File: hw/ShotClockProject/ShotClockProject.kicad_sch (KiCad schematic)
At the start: 5 parts, among them SW5 SW_SPDT

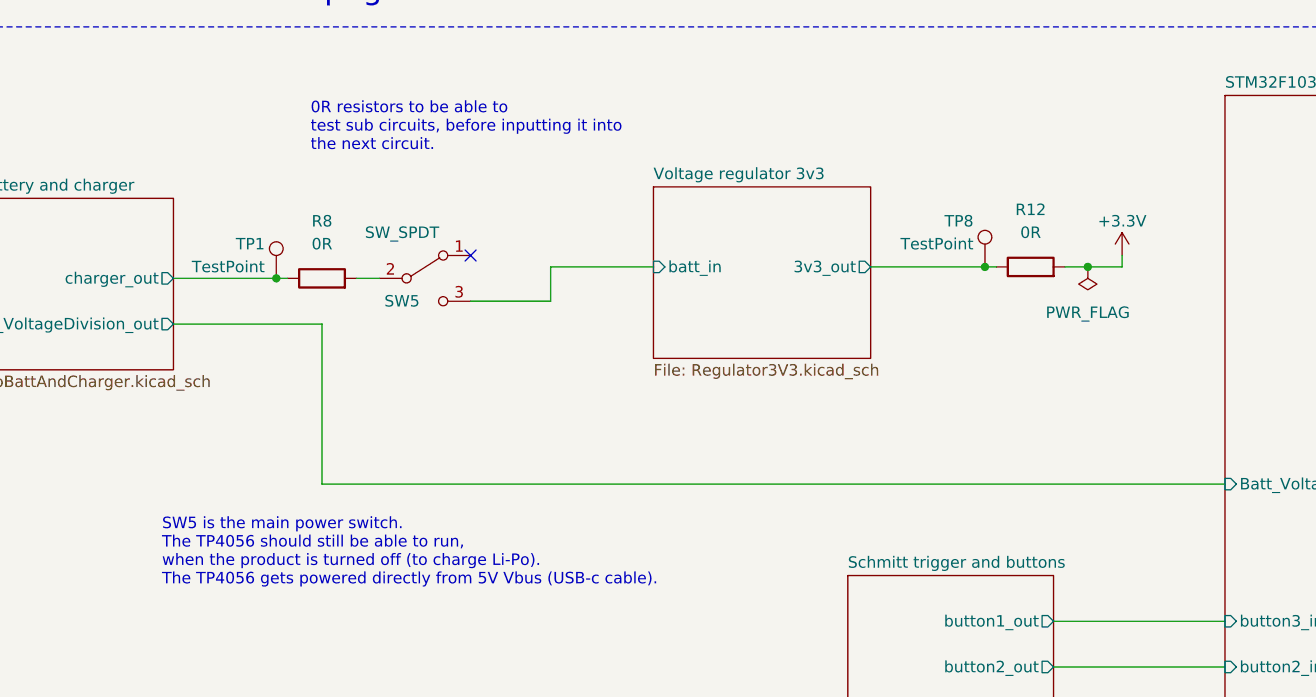
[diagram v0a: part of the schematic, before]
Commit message: Renamed references
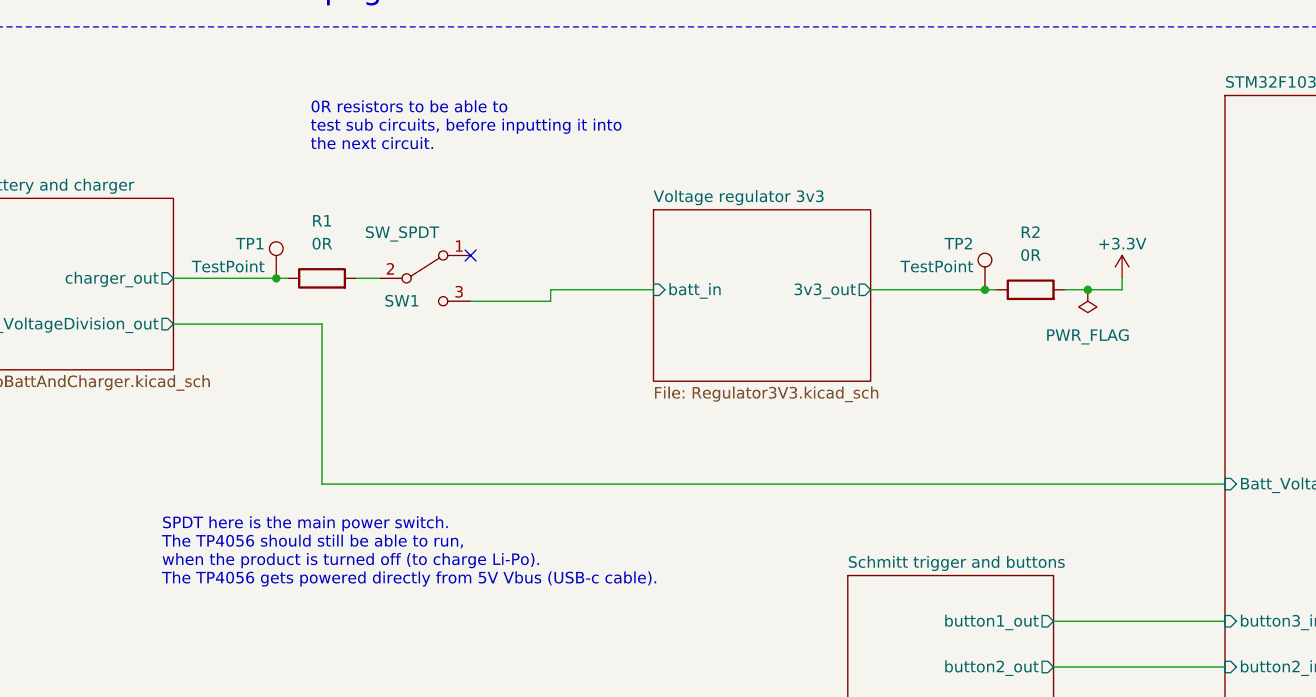
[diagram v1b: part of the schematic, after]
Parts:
- renumbered R8 to R1, R12 to R2, SW5 to SW1, TP8 to TP2
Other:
- note added: "SPDT here is the main power switch. The TP4056 should still be able to run, when the product is turned off (to charge Li-Po). The TP4056 gets powered directly from 5V Vbus (USB-c cable)."
- note removed: "SW5 is the main power switch. The TP4056 should still be able to run, when the product is turned off (to charge Li-Po). The TP4056 gets powered directly from 5V Vbus (USB-c cable)."
- moved on the sheet: R2, TP2
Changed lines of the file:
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@@
   (junction (at 59.69 49.53) (diameter 0) (color 0 0 0 0)
   )
-  (junction (at 149.86 48.26) (diameter 0) (color 0 0 0 0)
-  )
-  (junction (at 138.43 48.26) (diameter 0) (color 0 0 0 0)
+  (junction (at 149.86 50.8) (diameter 0) (color 0 0 0 0)
+  )
+  (junction (at 138.43 50.8) (diameter 0) (color 0 0 0 0)
   )
   (no_connect (at 81.28 46.99))
@@
     (stroke (width 0) (type default))
   )
-  (wire (pts (xy 138.43 48.26) (xy 139.7 48.26))
+  (wire (pts (xy 138.43 50.8) (xy 139.7 50.8))
     (stroke (width 0) (type default))
   )
@@
     (stroke (width 0) (type default))
   )
-  (wire (pts (xy 90.17 48.26) (xy 101.6 48.26))
+  (wire (pts (xy 90.17 50.8) (xy 90.17 52.07))
     (stroke (width 0) (type default))
   )
@@
     (stroke (width 0) (type default))
   )
-  (wire (pts (xy 125.73 48.26) (xy 138.43 48.26))
+  (wire (pts (xy 125.73 50.8) (xy 138.43 50.8))
     (stroke (width 0) (type default))
   )
@@
     (stroke (width 0) (type default))
   )
-  (wire (pts (xy 153.67 48.26) (xy 153.67 46.99))
+  (wire (pts (xy 153.67 50.8) (xy 153.67 49.53))
     (stroke (width 0) (type default))
   )
@@
     (stroke (width 0) (type default))
   )
-  (wire (pts (xy 147.32 48.26) (xy 149.86 48.26))
+  (wire (pts (xy 147.32 50.8) (xy 149.86 50.8))
     (stroke (width 0) (type default))
   )
@@
     (stroke (width 0) (type default))
   )
-  (wire (pts (xy 90.17 52.07) (xy 90.17 48.26))
-    (stroke (width 0) (type default))
-  )
   (wire (pts (xy 203.2 78.74) (xy 231.14 78.74))
     (stroke (width 0) (type default))
   )
-  (wire (pts (xy 149.86 48.26) (xy 153.67 48.26))
+  (wire (pts (xy 149.86 50.8) (xy 153.67 50.8))
+    (stroke (width 0) (type default))
+  )
+  (wire (pts (xy 101.6 50.8) (xy 90.17 50.8))
     (stroke (width 0) (type default))
   )
@@
     (effects (font (size 2.5 2.5) (color 255 0 0 1)) (justify left bottom))
   )
-  (text "SW5 is the main power switch.\nThe TP4056 should still be able to run, \nwhen the product is turned off (to charge Li-Po).\nThe TP4056 gets powered directly from 5V Vbus (USB-c cable)."
+  (text "SPDT here is the main power switch.\nThe TP4056 should still be able to run, \nwhen the product is turned off (to charge Li-Po).\nThe TP4056 gets powered directly from 5V Vbus (USB-c cable)."
     (at 46.99 83.82 0)
     (effects (font (size 1.27 1.27)) (justify left bottom))
@@
   (symbol (lib_id "Switch:SW_SPDT") (at 76.2 49.53 0) (unit 1)
     (in_bom yes) (on_board yes) (dnp no)
-    (property "Reference" "SW5" (at 73.66 52.07 0)
+    (property "Reference" "SW1" (at 73.66 52.07 0)
       (effects (font (size 1.27 1.27)))
     )
@@
       (project "ShotClockProject"
         (path "/5fd859aa-754d-49c2-9762-3f7ebe3bb64c"
-          (reference "SW5") (unit 1)
+          (reference "SW1") (unit 1)
         )
         (path "/5fd859aa-754d-49c2-9762-3f7ebe3bb64c/d53b1cd8-24cb-4dc0-9a02-0cd96c1f4291"
@@
   (symbol (lib_id "Device:R") (at 64.77 49.53 90) (unit 1)
     (in_bom yes) (on_board yes) (dnp no) (fields_autoplaced)
-    (property "Reference" "R8" (at 64.77 43.18 90)
+    (property "Reference" "R1" (at 64.77 43.18 90)
       (effects (font (size 1.27 1.27)))
     )
@@
       (project "ShotClockProject"
         (path "/5fd859aa-754d-49c2-9762-3f7ebe3bb64c"
-          (reference "R8") (unit 1)
-        )
-      )
-    )
-  )
-  (symbol (lib_id "Connector:TestPoint") (at 138.43 48.26 0) (mirror y) (unit 1)
+          (reference "R1") (unit 1)
+        )
+      )
+    )
+  )
+  (symbol (lib_id "Connector:TestPoint") (at 138.43 50.8 0) (mirror y) (unit 1)
     (in_bom yes) (on_board yes) (dnp no)
-    (property "Reference" "TP8" (at 137.16 43.18 0)
-      (effects (font (size 1.27 1.27)) (justify left))
-    )
-    (property "Value" "TestPoint" (at 137.16 45.72 0)
-      (effects (font (size 1.27 1.27)) (justify left))
-    )
-    (property "Footprint" "TestPoint:TestPoint_Pad_D2.5mm" (at 133.35 48.26 0)
-      (effects (font (size 1.27 1.27)) hide)
-    )
-    (property "Datasheet" "~" (at 133.35 48.26 0)
-      (effects (font (size 1.27 1.27)) hide)
-    )
-    (pin "1")
-    (instances
-      (project "ShotClockProject"
-        (path "/5fd859aa-754d-49c2-9762-3f7ebe3bb64c"
-          (reference "TP8") (unit 1)
+    (property "Reference" "TP2" (at 137.16 45.72 0)
+      (effects (font (size 1.27 1.27)) (justify left))
+    )
+    (property "Value" "TestPoint" (at 137.16 48.26 0)
+      (effects (font (size 1.27 1.27)) (justify left))
+    )
+    (property "Footprint" "TestPoint:TestPoint_Pad_D2.5mm" (at 133.35 50.8 0)
+      (effects (font (size 1.27 1.27)) hide)
+    )
+    (property "Datasheet" "~" (at 133.35 50.8 0)
+      (effects (font (size 1.27 1.27)) hide)
+    )
+    (pin "1")
+    (instances
+      (project "ShotClockProject"
+        (path "/5fd859aa-754d-49c2-9762-3f7ebe3bb64c"
+          (reference "TP2") (unit 1)
         )
         (path "/5fd859aa-754d-49c2-9762-3f7ebe3bb64c/17367eb9-0f4d-4017-b1ca-d50430410a5d"
@@
     )
   )
-  (symbol (lib_id "Device:R") (at 143.51 48.26 90) (unit 1)
+  (symbol (lib_id "Device:R") (at 143.51 50.8 90) (unit 1)
     (in_bom yes) (on_board yes) (dnp no) (fields_autoplaced)
-    (property "Reference" "R12" (at 143.51 41.91 90)
-      (effects (font (size 1.27 1.27)))
-    )
-    (property "Value" "0R" (at 143.51 44.45 90)
-      (effects (font (size 1.27 1.27)))
-    )
-    (property "Footprint" "Resistor_SMD:R_0603_1608Metric" (at 143.51 50.038 90)
-      (effects (font (size 1.27 1.27)) hide)
-    )
-    (property "Datasheet" "~" (at 143.51 48.26 0)
+    (property "Reference" "R2" (at 143.51 44.45 90)
+      (effects (font (size 1.27 1.27)))
+    )
+    (property "Value" "0R" (at 143.51 46.99 90)
+      (effects (font (size 1.27 1.27)))
+    )
+    (property "Footprint" "Resistor_SMD:R_0603_1608Metric" (at 143.51 52.578 90)
+      (effects (font (size 1.27 1.27)) hide)
+    )
+    (property "Datasheet" "~" (at 143.51 50.8 0)
       (effects (font (size 1.27 1.27)) hide)
     )
@@
       (project "ShotClockProject"
         (path "/5fd859aa-754d-49c2-9762-3f7ebe3bb64c"
-          (reference "R12") (unit 1)
-        )
-      )
-    )
-  )
-  (symbol (lib_id "power:PWR_FLAG") (at 149.86 48.26 180) (unit 1)
+          (reference "R2") (unit 1)
+        )
+      )
+    )
+  )
+  (symbol (lib_id "power:PWR_FLAG") (at 149.86 50.8 180) (unit 1)
     (in_bom yes) (on_board yes) (dnp no) (fields_autoplaced)
-    (property "Reference" "#FLG02" (at 149.86 50.165 0)
-      (effects (font (size 1.27 1.27)) hide)
-    )
-    (property "Value" "PWR_FLAG" (at 149.86 53.34 0)
-      (effects (font (size 1.27 1.27)))
-    )
-    (property "Footprint" "" (at 149.86 48.26 0)
-      (effects (font (size 1.27 1.27)) hide)
-    )
-    (property "Datasheet" "~" (at 149.86 48.26 0)
+    (property "Reference" "#FLG02" (at 149.86 52.705 0)
+      (effects (font (size 1.27 1.27)) hide)
+    )
+    (property "Value" "PWR_FLAG" (at 149.86 55.88 0)
+      (effects (font (size 1.27 1.27)))
+    )
+    (property "Footprint" "" (at 149.86 50.8 0)
+      (effects (font (size 1.27 1.27)) hide)
+    )
+    (property "Datasheet" "~" (at 149.86 50.8 0)
       (effects (font (size 1.27 1.27)) hide)
     )
@@
         )
         (path "/5fd859aa-754d-49c2-9762-3f7ebe3bb64c"
-          (reference "#FLG03") (unit 1)
-        )
-      )
-    )
-  )
-  (symbol (lib_id "power:+3.3V") (at 153.67 46.99 0) (unit 1)
+          (reference "#FLG01") (unit 1)
+        )
+      )
+    )
+  )
+  (symbol (lib_id "power:+3.3V") (at 153.67 49.53 0) (unit 1)
     (in_bom yes) (on_board yes) (dnp no)
-    (property "Reference" "#PWR033" (at 153.67 50.8 0)
-      (effects (font (size 1.27 1.27)) hide)
-    )
-    (property "Value" "+3.3V" (at 153.67 43.18 0)
-      (effects (font (size 1.27 1.27)))
-    )
-    (property "Footprint" "" (at 153.67 46.99 0)
-      (effects (font (size 1.27 1.27)) hide)
-    )
-    (property "Datasheet" "" (at 153.67 46.99 0)
-      (effects (font (size 1.27 1.27)) hide)
-    )
-    (pin "1")
-    (instances
-      (project "ShotClockProject"
-        (path "/5fd859aa-754d-49c2-9762-3f7ebe3bb64c"
-          (reference "#PWR033") (unit 1)
+    (property "Reference" "#PWR01" (at 153.67 53.34 0)
+      (effects (font (size 1.27 1.27)) hide)
+    )
+    (property "Value" "+3.3V" (at 153.67 45.72 0)
+      (effects (font (size 1.27 1.27)))
+    )
+    (property "Footprint" "" (at 153.67 49.53 0)
+      (effects (font (size 1.27 1.27)) hide)
+    )
+    (property "Datasheet" "" (at 153.67 49.53 0)
+      (effects (font (size 1.27 1.27)) hide)
+    )
+    (pin "1")
+    (instances
+      (project "ShotClockProject"
+        (path "/5fd859aa-754d-49c2-9762-3f7ebe3bb64c"
+          (reference "#PWR01") (unit 1)
         )
         (path "/5fd859aa-754d-49c2-9762-3f7ebe3bb64c/d53b1cd8-24cb-4dc0-9a02-0cd96c1f4291"
@@
     )
   )
-  (sheet (at 101.6 39.37) (size 24.13 19.05) (fields_autoplaced)
+  (sheet (at 101.6 41.91) (size 24.13 19.05) (fields_autoplaced)
     (stroke (width 0.1524) (type solid))
     (fill (color 0 0 0 0.0000))
-    (property "Sheetname" "Voltage regulator 3v3" (at 101.6 38.6584 0)
+    (property "Sheetname" "Voltage regulator 3v3" (at 101.6 41.1984 0)
       (effects (font (size 1.27 1.27)) (justify left bottom))
     )
-    (property "Sheetfile" "Regulator3V3.kicad_sch" (at 101.6 59.0046 0)
+    (property "Sheetfile" "Regulator3V3.kicad_sch" (at 101.6 61.5446 0)
       (effects (font (size 1.27 1.27)) (justify left top))
     )
-    (pin "batt_in" input (at 101.6 48.26 180)
-      (effects (font (size 1.27 1.27)) (justify left))
-    )
-    (pin "3v3_out" output (at 125.73 48.26 0)
+    (pin "batt_in" input (at 101.6 50.8 180)
+      (effects (font (size 1.27 1.27)) (justify left))
+    )
+    (pin "3v3_out" output (at 125.73 50.8 0)
       (effects (font (size 1.27 1.27)) (justify right))
     )
